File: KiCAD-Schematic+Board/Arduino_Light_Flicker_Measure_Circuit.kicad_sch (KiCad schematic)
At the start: 42 parts, among them J1 Ds, J2 Ds, J3 FTDI, J4 FTDI-Conn, J5 PWR(5V), J6 USB Power (5V), Q1 BC547, Q2 BC547, U1 ATmega328P-PU, U2 AD5242, U3 AD823A, U4 Display

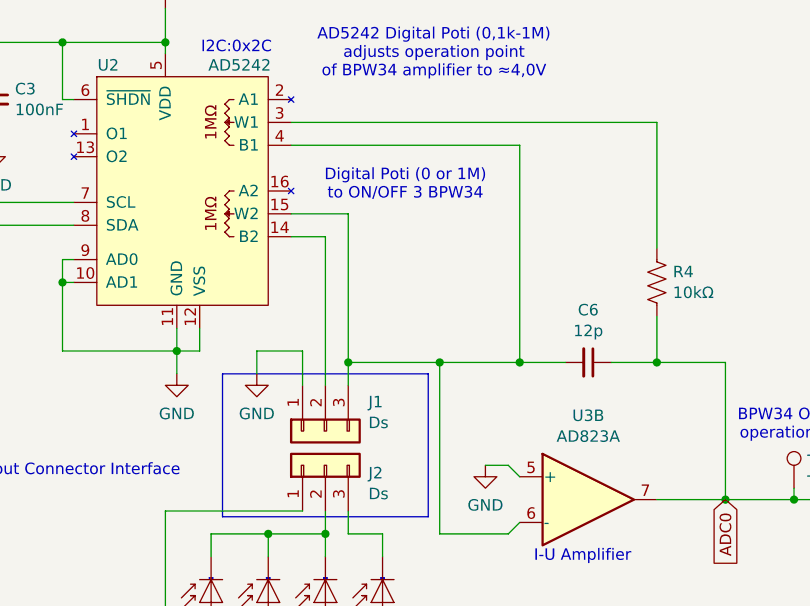
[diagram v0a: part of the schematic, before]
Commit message: Update to do basic messed-up layout.  Imperfect but hopefully functional.
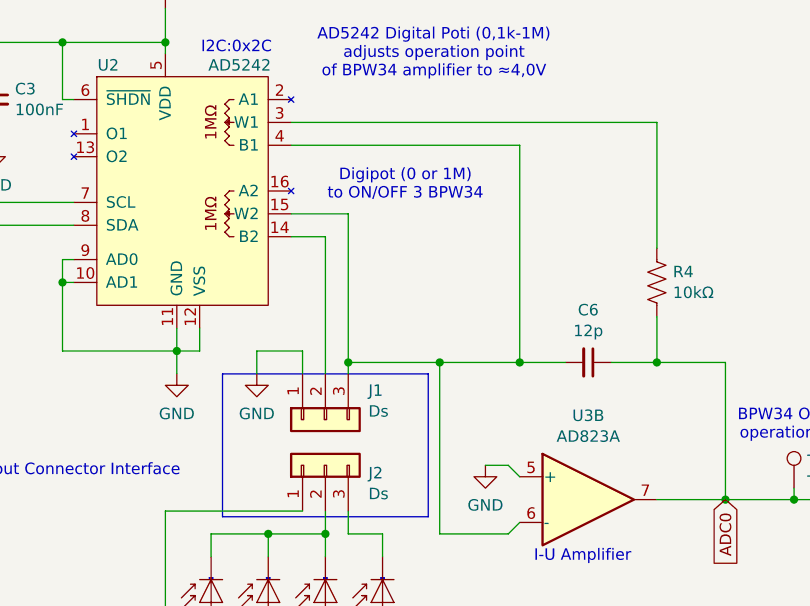
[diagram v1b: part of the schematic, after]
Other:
- note added: "Digipot (0 or 1M) to ON/OFF 3 BPW34"
- note removed: "Digital Poti (0 or 1M) to ON/OFF 3 BPW34"
- moved on the sheet: J1
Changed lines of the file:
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@@
     (stroke (width 0) (type default))
   )
-  (wire (pts (xy 77.47 62.23) (xy 77.47 66.04))
+  (wire (pts (xy 77.47 62.23) (xy 77.47 64.77))
     (stroke (width 0) (type default))
   )
@@
     (stroke (width 0) (type default))
   )
-  (wire (pts (xy 82.55 66.04) (xy 82.55 63.5))
+  (wire (pts (xy 82.55 64.77) (xy 82.55 63.5))
     (stroke (width 0) (type default))
   )
@@
     (stroke (width 0) (type default))
   )
-  (wire (pts (xy 80.01 49.53) (xy 80.01 66.04))
+  (wire (pts (xy 80.01 49.53) (xy 80.01 64.77))
     (stroke (width 0) (type default))
   )
@@
     (effects (font (size 1.27 1.27)))
   )
-  (text "Digital Poti (0 or 1M)\nto ON/OFF 3 BPW34\n" (exclude_from_sim no)
+  (text "Digipot (0 or 1M)\nto ON/OFF 3 BPW34\n" (exclude_from_sim no)
  (at 88.9 43.815 0)
     (effects (font (size 1.27 1.27)))
@@
     )
   )
-  (symbol (lib_id "Connector_Generic:Conn_01x03") (at 80.01 71.12 90) (mirror x) (unit 1)
-    (exclude_from_sim no) (in_bom yes) (on_board yes) (dnp no)
-    (property "Reference" "J1" (at 84.7852 67.8942 90)
+  (symbol (lib_id "Connector_Generic:Conn_01x03") (at 80.01 69.85 90) (mirror x) (unit 1)
+    (exclude_from_sim no) (in_bom yes) (on_board yes) (dnp no)
+    (property "Reference" "J1" (at 84.7852 66.6242 90)
       (effects (font (size 1.27 1.27)) (justify right))
     )
-    (property "Value" "Ds" (at 84.7852 70.2056 90)
+    (property "Value" "Ds" (at 84.7852 68.9356 90)
       (effects (font (size 1.27 1.27)) (justify right))
     )
-    (property "Footprint" "Connector_PinHeader_2.54mm:PinHeader_1x03_P2.54mm_Vertical" (at 80.01 71.12 0)
-      (effects (font (size 1.27 1.27)) hide)
-    )
-    (property "Datasheet" "~" (at 80.01 71.12 0)
-      (effects (font (size 1.27 1.27)) hide)
-    )
-    (property "Description" "" (at 80.01 71.12 0)
-      (effects (font (size 1.27 1.27)) hide)
-    )
+    (property "Footprint" "Connector_PinHeader_2.54mm:PinHeader_1x03_P2.54mm_Vertical" (at 80.01 69.85 0)
+      (effects (font (size 1.27 1.27)) hide)
+    )
+    (property "Datasheet" "~" (at 80.01 69.85 0)
+      (effects (font (size 1.27 1.27)) hide)
+    )
+    (property "Description" "" (at 80.01 69.85 0)
+      (effects (font (size 1.27 1.27)) hide)
+    )
